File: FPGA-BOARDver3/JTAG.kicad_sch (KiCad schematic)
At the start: 23 parts, among them J6 Conn_01x06_Pin, U1 XC7Z020-1CLG400I__, U34 TPD4E05U06DQAR, U4 ATSHA204A-SSHCZ-T, U7 S25FL128SAGMFI000

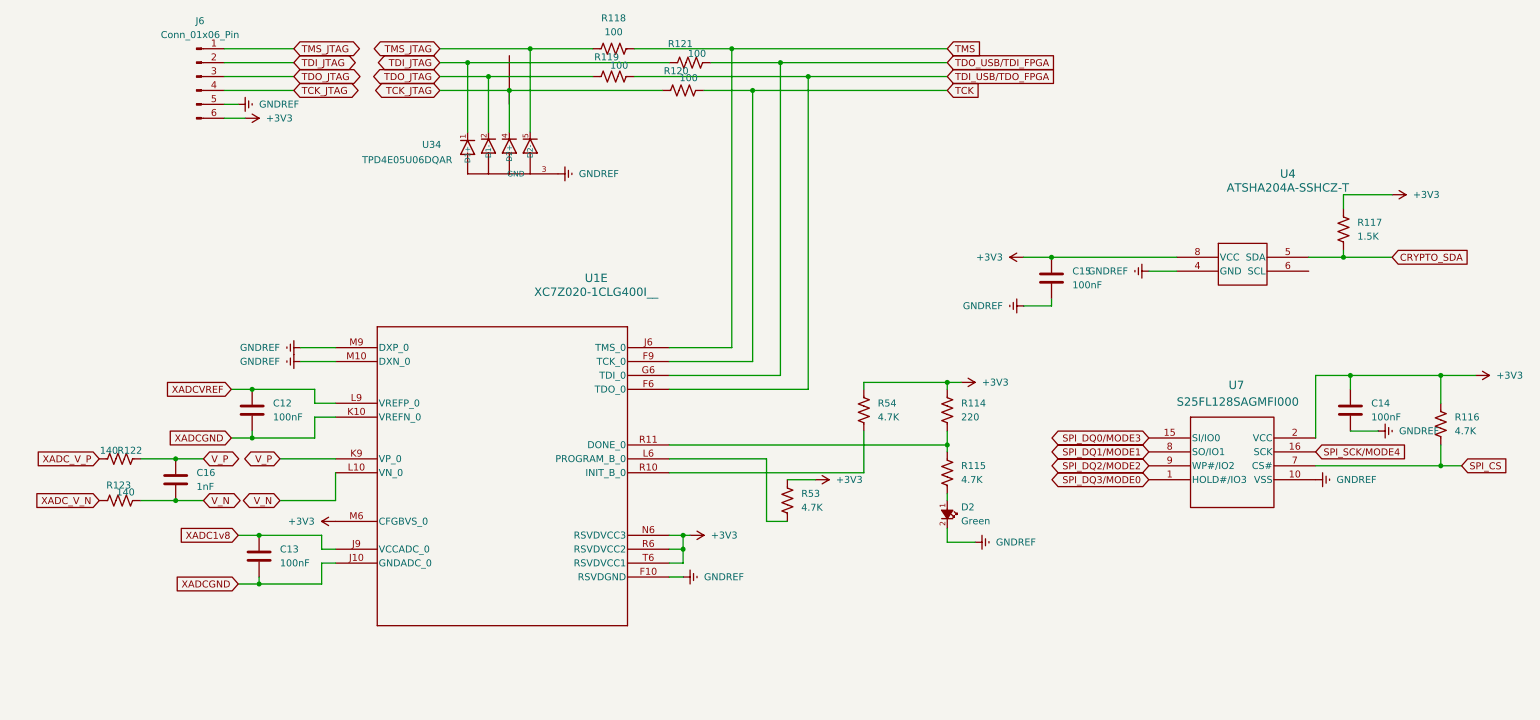
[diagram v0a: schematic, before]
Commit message: updated schematic and layout
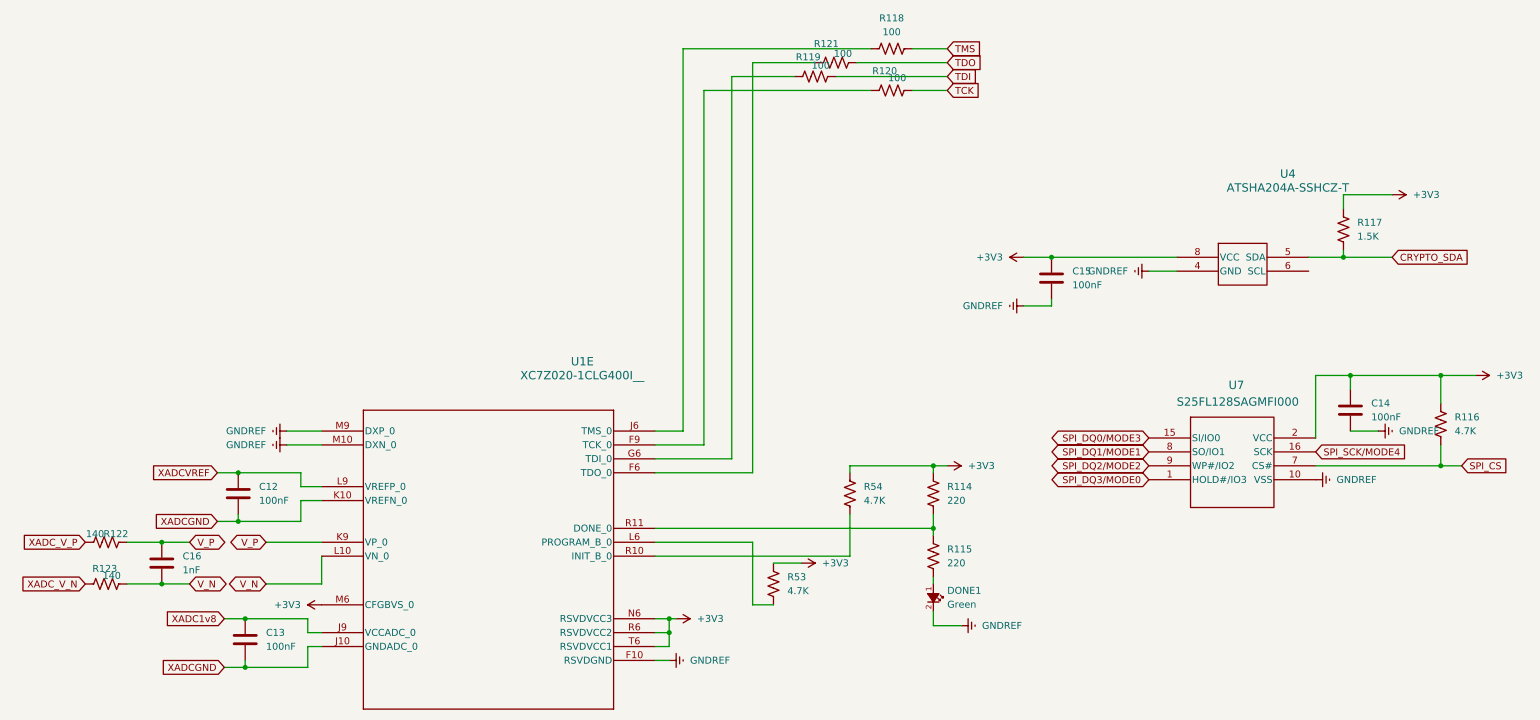
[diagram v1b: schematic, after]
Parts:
- removed J6: Conn_01x06_Pin, footprints:CONN6_PZ254V-11-06P_XFC, symbol Connector:Conn_01x06_Pin
- removed U34: TPD4E05U06DQAR, footprints:IC_TPD4E05U06DQAR, symbol TPD4E05U06DQAR:TPD4E05U06DQAR
- C12, C13, C14, C15: LCSC PN (none) -> c1525
- C16: LCSC PN (none) -> c14442
- DONE1: renamed from D2; LCSC PN (none) -> C434449
- R114: LCSC PN (none) -> C112291
- R115: value 4.7K -> 220; LCSC PN (none) -> C112291
- R116, R53, R54: LCSC PN (none) -> C105871
- R117: LCSC PN (none) -> C114759
- R118, R119, R120, R121: LCSC PN (none) -> C106232
- R122, R123: LCSC PN (none) -> C327016
- U1: LCSC PN (none) -> C1519081
- U4: LCSC PN (none) -> C616025
- U7: LCSC PN (none) -> C393875
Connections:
- net TCK: no longer U1.F9 (TCK_0)
- net TMS: no longer U1.J6 (TMS_0)
- net TCK_JTAG: no longer names the net of R120.1
- net TCK_JTAG: now also U1.F9 (TCK_0)
- net TDI_JTAG: no longer names the net of R121.1
- net TDI_JTAG: now also U1.F6 (TDO_0)
- net TDI_USB/TDO_FPGA renamed TDI
- net TDI: no longer U1.F6 (TDO_0)
- net TDO_JTAG: no longer names the net of R119.1
- net TDO_JTAG: now also U1.G6 (TDI_0)
- net TDO_USB/TDI_FPGA renamed TDO
- net TDO: no longer U1.G6 (TDI_0)
- net TMS_JTAG: no longer names the net of R118.1
- net TMS_JTAG: now also U1.J6 (TMS_0)
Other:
- moved on the sheet: C12, C13, C16, DONE1, R114, R115, R118, R119, R120, R121, R122, R123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
